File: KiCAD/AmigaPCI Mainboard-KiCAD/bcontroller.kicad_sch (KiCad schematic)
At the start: 20 parts, among them CN227 JTAG/SWD, J200 DISABLE AUTOBOOT, U6 XC95144XL-TQ144, U711 XC9572XL-VQ64

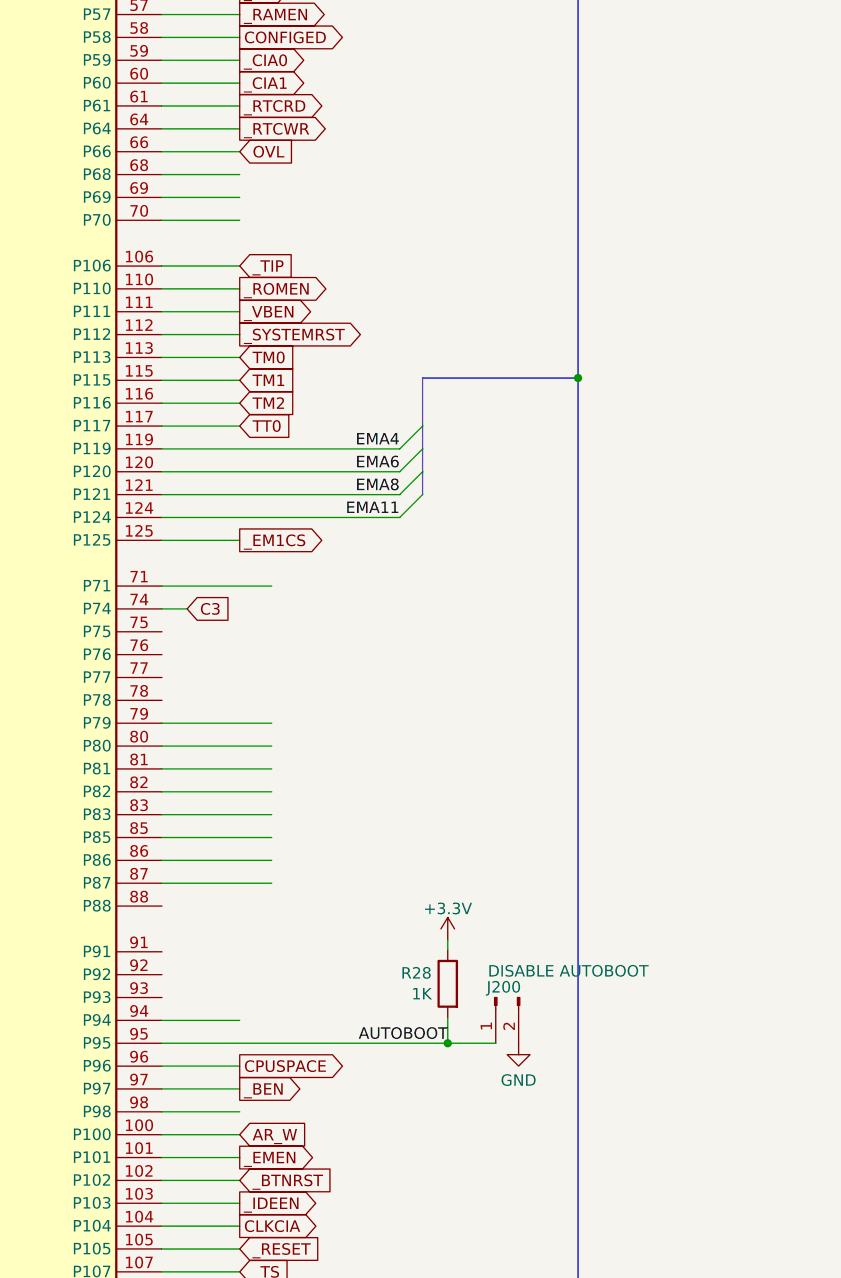
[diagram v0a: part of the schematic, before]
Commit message: Routing 21-DEC-2023
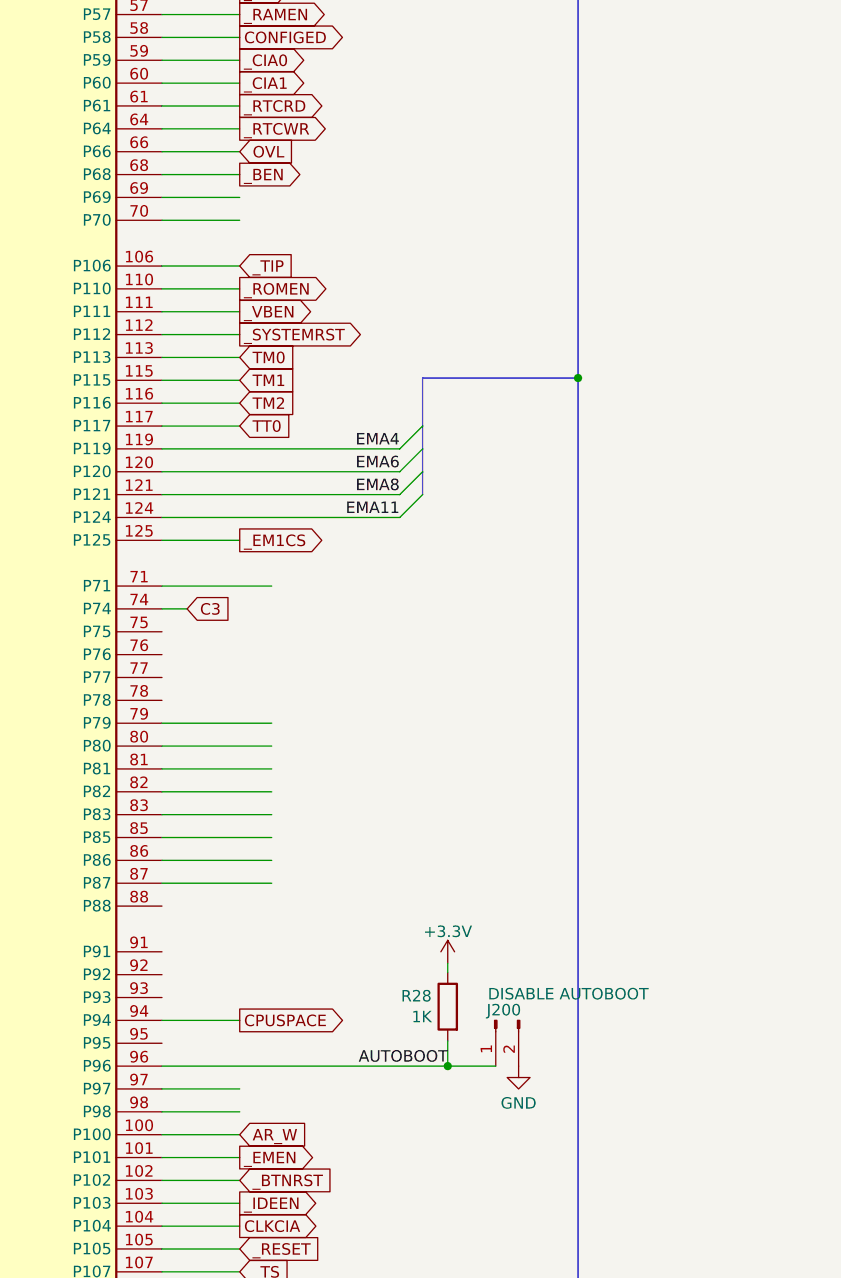
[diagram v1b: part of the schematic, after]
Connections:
- net AUTOBOOT: now also U6.96 (P96); no longer U6.95 (P95)
- net CPUSPACE: now also U6.94 (P94); no longer U6.96 (P96)
- net _BEN: now also U6.68 (P68); no longer U6.97 (P97)
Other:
- moved on the sheet: J200, R28
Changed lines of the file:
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@@
   (junction (at 168.402 46.736) (diameter 0) (color 0 0 0 0)
   )
-  (junction (at 210.566 195.072) (diameter 0) (color 0 0 0 0)
+  (junction (at 210.566 197.612) (diameter 0) (color 0 0 0 0)
   )
   (junction (at 332.232 75.946) (diameter 0) (color 0 0 0 0)
@@
     (stroke (width 0) (type default))
   )
-  (wire (pts (xy 215.9 195.072) (xy 210.566 195.072))
+  (wire (pts (xy 215.9 197.612) (xy 210.566 197.612))
     (stroke (width 0) (type default))
   )
@@
     (stroke (width 0) (type default))
   )
-  (wire (pts (xy 210.566 183.642) (xy 210.566 184.658))
+  (wire (pts (xy 210.566 186.182) (xy 210.566 187.198))
     (stroke (width 0) (type default))
   )
@@
     (stroke (width 0) (type default))
   )
-  (wire (pts (xy 187.452 197.612) (xy 178.816 197.612))
-    (stroke (width 0) (type default))
-  )
   (wire (pts (xy 153.416 46.736) (xy 150.876 46.736))
     (stroke (width 0) (type default))
@@
     (stroke (width 0) (type default))
   )
-  (wire (pts (xy 210.566 195.072) (xy 178.816 195.072))
+  (wire (pts (xy 210.566 197.612) (xy 178.816 197.612))
     (stroke (width 0) (type default))
   )
@@
     (stroke (width 0) (type default))
   )
-  (wire (pts (xy 210.566 192.278) (xy 210.566 195.072))
+  (wire (pts (xy 210.566 194.818) (xy 210.566 197.612))
     (stroke (width 0) (type default))
   )
@@
     (effects (font (size 1.27 1.27)) (justify left bottom))
   )
-  (label "AUTOBOOT" (at 210.566 195.072 180) (fields_autoplaced)
+  (label "AUTOBOOT" (at 210.566 197.612 180) (fields_autoplaced)
     (effects (font (size 1.27 1.27)) (justify right bottom))
   )
@@
     )
   )
-  (global_label "_BEN" (shape output) (at 187.452 200.152 0) (fields_autoplaced)
-    (effects (font (size 1.27 1.27)) (justify left))
-    (property "Intersheetrefs" "${INTERSHEET_REFS}" (at 195.0749 200.152 0)
+  (global_label "_BEN" (shape output) (at 187.452 98.552 0) (fields_autoplaced)
+    (effects (font (size 1.27 1.27)) (justify left))
+    (property "Intersheetrefs" "${INTERSHEET_REFS}" (at 195.0749 98.552 0)
       (effects (font (size 1.27 1.27)) (justify left))
     )
@@
     )
   )
-  (global_label "CPUSPACE" (shape output) (at 187.452 197.612 0) (fields_autoplaced)
-    (effects (font (size 1.27 1.27)) (justify left))
-    (property "Intersheetrefs" "${INTERSHEET_REFS}" (at 200.2154 197.612 0)
+  (global_label "CPUSPACE" (shape output) (at 187.452 192.532 0) (fields_autoplaced)
+    (effects (font (size 1.27 1.27)) (justify left))
+    (property "Intersheetrefs" "${INTERSHEET_REFS}" (at 200.2154 192.532 0)
       (effects (font (size 1.27 1.27)) (justify left))
     )
@@
     )
   )
-  (symbol (lib_id "power:+3.3V") (at 210.566 183.642 0) (mirror y) (unit 1)
+  (symbol (lib_id "power:+3.3V") (at 210.566 186.182 0) (mirror y) (unit 1)
     (in_bom yes) (on_board yes) (dnp no) (fields_autoplaced)
-    (property "Reference" "#PWR05" (at 210.566 187.452 0)
-      (effects (font (size 1.27 1.27)) hide)
-    )
-    (property "Value" "+3.3V" (at 210.566 180.1401 0)
+    (property "Reference" "#PWR05" (at 210.566 189.992 0)
+      (effects (font (size 1.27 1.27)) hide)
+    )
+    (property "Value" "+3.3V" (at 210.566 182.6801 0)
       (effects (font (size 1.27 1.27)))
     )
-    (property "Footprint" "" (at 210.566 183.642 0)
-      (effects (font (size 1.27 1.27)) hide)
-    )
-    (property "Datasheet" "" (at 210.566 183.642 0)
+    (property "Footprint" "" (at 210.566 186.182 0)
+      (effects (font (size 1.27 1.27)) hide)
+    )
+    (property "Datasheet" "" (at 210.566 186.182 0)
       (effects (font (size 1.27 1.27)) hide)
     )
@@
     )
   )
-  (symbol (lib_id "Device:R") (at 210.566 188.468 0) (mirror y) (unit 1)
+  (symbol (lib_id "Device:R") (at 210.566 191.008 0) (mirror y) (unit 1)
     (in_bom yes) (on_board yes) (dnp no)
-    (property "Reference" "R28" (at 208.788 187.2996 0)
-      (effects (font (size 1.27 1.27)) (justify left))
-    )
-    (property "Value" "1K" (at 208.788 189.611 0)
-      (effects (font (size 1.27 1.27)) (justify left))
-    )
-    (property "Footprint" "Resistor_SMD:R_0603_1608Metric" (at 212.344 188.468 90)
-      (effects (font (size 1.27 1.27)) hide)
-    )
-    (property "Datasheet" "~" (at 210.566 188.468 0)
+    (property "Reference" "R28" (at 208.788 189.8396 0)
+      (effects (font (size 1.27 1.27)) (justify left))
+    )
+    (property "Value" "1K" (at 208.788 192.151 0)
+      (effects (font (size 1.27 1.27)) (justify left))
+    )
+    (property "Footprint" "Resistor_SMD:R_0603_1608Metric" (at 212.344 191.008 90)
+      (effects (font (size 1.27 1.27)) hide)
+    )
+    (property "Datasheet" "~" (at 210.566 191.008 0)
       (effects (font (size 1.27 1.27)) hide)
     )
@@
     )
   )
-  (symbol (lib_id "power:GND") (at 218.44 195.072 0) (mirror y) (unit 1)
+  (symbol (lib_id "power:GND") (at 218.44 197.612 0) (mirror y) (unit 1)
     (in_bom yes) (on_board yes) (dnp no) (fields_autoplaced)
-    (property "Reference" "#PWR0243" (at 218.44 201.422 0)
-      (effects (font (size 1.27 1.27)) hide)
-    )
-    (property "Value" "GND" (at 218.44 199.2075 0)
+    (property "Reference" "#PWR0243" (at 218.44 203.962 0)
+      (effects (font (size 1.27 1.27)) hide)
+    )
+    (property "Value" "GND" (at 218.44 201.7475 0)
       (effects (font (size 1.27 1.27)))
     )
-    (property "Footprint" "" (at 218.44 195.072 0)
-      (effects (font (size 1.27 1.27)) hide)
-    )
-    (property "Datasheet" "" (at 218.44 195.072 0)
+    (property "Footprint" "" (at 218.44 197.612 0)
+      (effects (font (size 1.27 1.27)) hide)
+    )
+    (property "Datasheet" "" (at 218.44 197.612 0)
       (effects (font (size 1.27 1.27)) hide)
     )
@@
     )
   )
-  (symbol (lib_id "Connector:Conn_01x02_Pin") (at 215.9 189.992 90) (mirror x) (unit 1)
+  (symbol (lib_id "Connector:Conn_01x02_Pin") (at 215.9 192.532 90) (mirror x) (unit 1)
     (in_bom yes) (on_board yes) (dnp no)
-    (property "Reference" "J200" (at 214.884 188.849 90)
-      (effects (font (size 1.27 1.27)) (justify right))
-    )
-    (property "Value" "DISABLE AUTOBOOT" (at 215.011 187.071 90)
-      (effects (font (size 1.27 1.27)) (justify right))
-    )
-    (property "Footprint" "Connector_PinHeader_2.54mm:PinHeader_1x02_P2.54mm_Vertical" (at 215.9 189.992 0)
-      (effects (font (size 1.27 1.27)) hide)
-    )
-    (property "Datasheet" "~" (at 215.9 189.992 0)
-      (effects (font (size 1.27 1.27)) hide)
-    )
+    (property "Reference" "J200" (at 214.884 191.389 90)
+      (effects (font (size 1.27 1.27)) (justify right))
+    )
+    (property "Value" "DISABLE AUTOBOOT" (at 215.011 189.611 90)
+      (effects (font (size 1.27 1.27)) (justify right))
+    )
+    (property "Footprint" "Connector_PinHeader_2.54mm:PinHeader_1x02_P2.54mm_Vertical" (at 215.9 192.532 0)
+      (effects (font (size 1.27 1.27)) hide)
+    )
+    (property "Datasheet" "~" (at 215.9 192.532 0)
+      (effects (font (size 1.27 1.27)) hide)
+    )
